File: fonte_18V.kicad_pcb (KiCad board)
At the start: 2 copper layers, 100 x 52 mm, 35 parts, among them J1 MSTBA, J2 MSTBA, J3 RJ45_Shielded, J4 RJ45_Shielded, Q1 Si2308CDS, U1 LMR16030

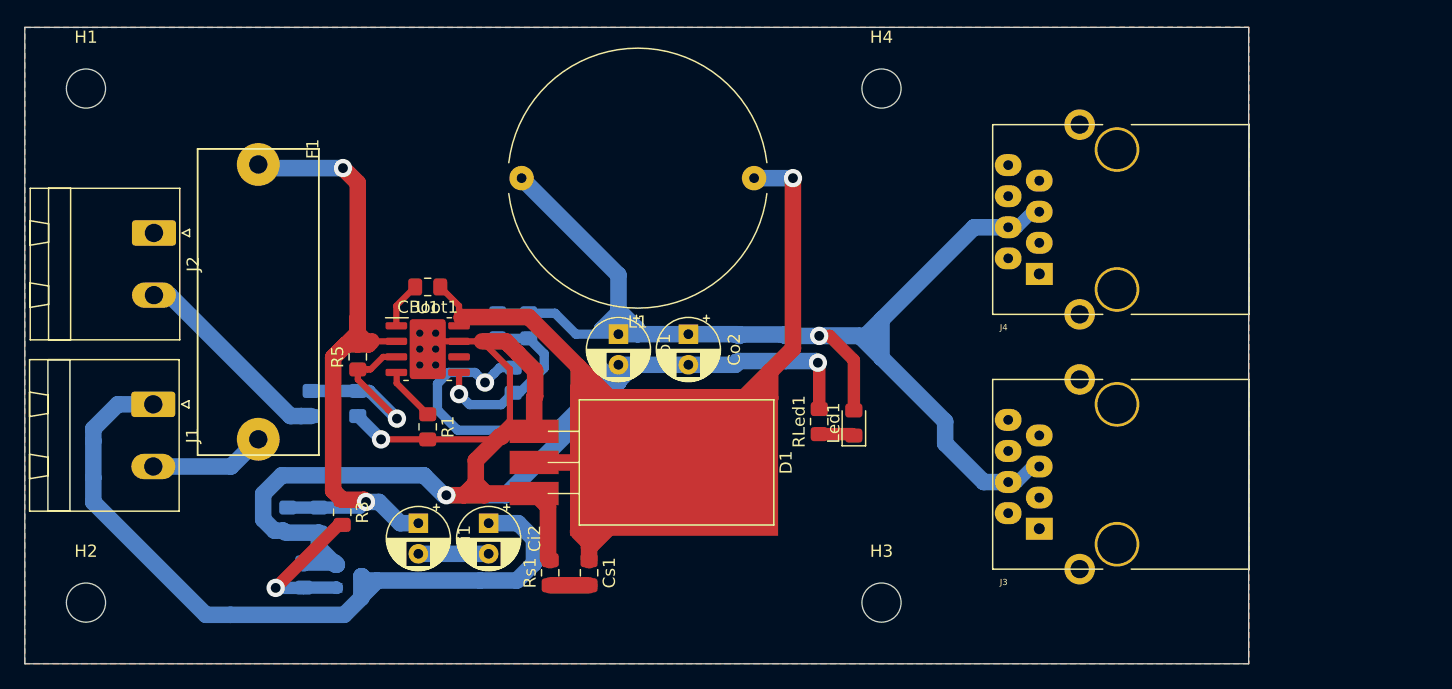
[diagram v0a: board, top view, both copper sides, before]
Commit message: temp
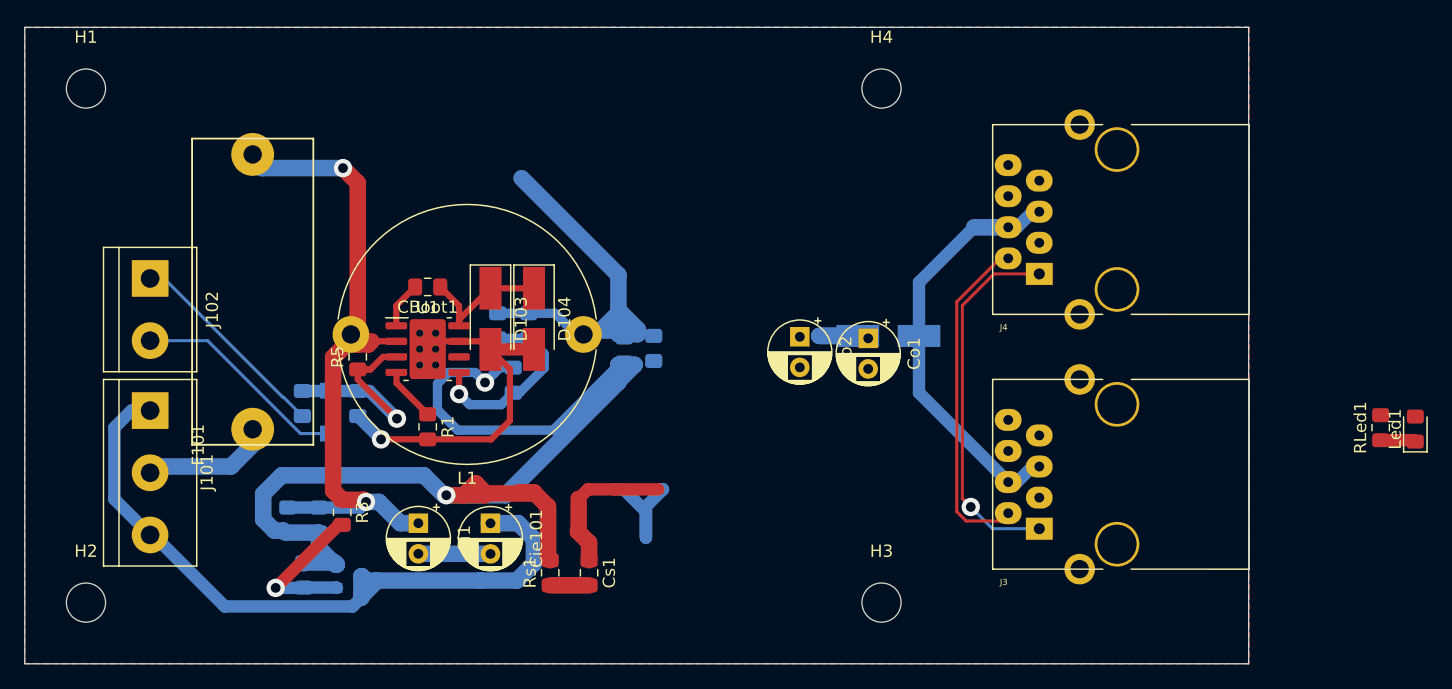
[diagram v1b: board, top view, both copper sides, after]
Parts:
- removed Ci2: 10u, Capacitor_THT:CP_Radial_D5.0mm_P2.50mm
- removed D1: MBR20200CTG, Package_TO_SOT_THT:TO-220-3_Horizontal_TabDown_SMD
- removed F1: 2A, KicadZeniteSolarLibrary18:Fuse_Holder_5x20
- removed J1, J2: MSTBA, Connector_Phoenix_MSTB:PhoenixContact_MSTBA_2,5_2-G-5,08_1x02_P5.08mm_Horizontal
- added Cie101: 10u, Capacitor_THT:CP_Radial_D5.0mm_P2.50mm, F.Cu at (60.5, 176.7)
- added D101: 4v7, Diode_SMD:D_MiniMELF, B.Cu at (47.4, 167.6)
- added D102: MBR340, Diode_SMD:D_SMA_Handsoldering, B.Cu at (93.0, 161.4)
- added D103: B1100, Diode_SMD:D_SMA_Handsoldering, F.Cu at (60.5, 160.0)
- added D104: B1100, Diode_SMD:D_SMA_Handsoldering, F.Cu at (64.0, 160.0)
- added F101: Fuse, KicadZeniteSolarLibrary18:Fuse_Holder_5x20, F.Cu at (36.1, 170.3)
- added J101: IN, TerminalBlock:TerminalBlock_bornier-3_P5.08mm, F.Cu at (32.6, 167.5)
- added J102: Conn_01x02, TerminalBlock:TerminalBlock_bornier-2_P5.08mm, F.Cu at (32.6, 156.7)
- R2: value 100 -> 1k
- moved RLed1 45.9 mm to (133.2, 168.9)
- moved Led1 45.9 mm to (136.0, 169.0)
- moved Co1 20.4 mm to (91.3, 161.6)
- moved L1 18.9 mm to (68.0, 161.3)
- moved Co3 10.8 mm to (73.8, 162.4)
- moved Co4 9.39 mm to (71.4, 162.6)
- moved Co2 9.11 mm to (85.7, 161.5)
- moved R2 0.71 mm to (45.1, 166.9)
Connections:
- net Net-(R2-Pad1) renamed /EN
- Cff1 pad 1: /CAN_18V -> /CAN_18V_DIODE
- Co1 pad 1: /CAN_18V -> /CAN_18V_DIODE
- Co2 pad 1: /CAN_18V -> /CAN_18V_DIODE
- Co3 pad 1: /CAN_18V -> /CAN_18V_DIODE
- Co4 pad 1: /CAN_18V -> /CAN_18V_DIODE
- J3 pad 1: (no net) -> Net-(J4-Pad1)
- J3 pad 2: (no net) -> Net-(J4-Pad2)
- J3 pad 9: GND -> (no net)
- J4 pad 1: (no net) -> Net-(J4-Pad1)
- J4 pad 2: (no net) -> Net-(J4-Pad2)
- J4 pad 9: GND -> (no net)
- L1 pad 2: /CAN_18V -> /CAN_18V_DIODE
- Led1 pad 2: /CAN_18V -> /CAN_18V_DIODE
- Rfbt2 pad 1: /CAN_18V -> /CAN_18V_DIODE
- U1 pad 6: (no net) -> unconnected-(U1-Pad6)
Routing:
- net /CAN_18V: track 108.7 -> 34.6 mm, vias 1 -> 0
- net Net-(CBoot1-Pad1): track 98.6 -> 34.1 mm, vias 1 -> 0
- net /CAN_18V_DIODE: track 0.00 -> 43.1 mm
- net Net-(J4-Pad1): track 0.00 -> 30.4 mm, vias 0 -> 1
- net Net-(J4-Pad2): track 0.00 -> 27.6 mm
- net GND: track 167.3 -> 147.9 mm, vias 4 -> 3
- net Net-(J101-Pad2): track 0.00 -> 9.50 mm
- net Net-(F1-Pad2): track 9.50 -> 0.00 mm
- net Net-(Cie101-Pad1): track 62.8 -> 58.2 mm
